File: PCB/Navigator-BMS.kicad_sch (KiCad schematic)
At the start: 49 parts, among them IC1 AP2112K, J1 Conn_01x03, J2 CAN, J3 CAN, J4 Conn_01x05, Q1 IRF7480M, U1 BQ76920PW, U2 MCP2551-I-SN, U3 TMP117xxDRV, U4 STM32G441KBUx, U5 SN74AUP1T34DCK, U6 TPS

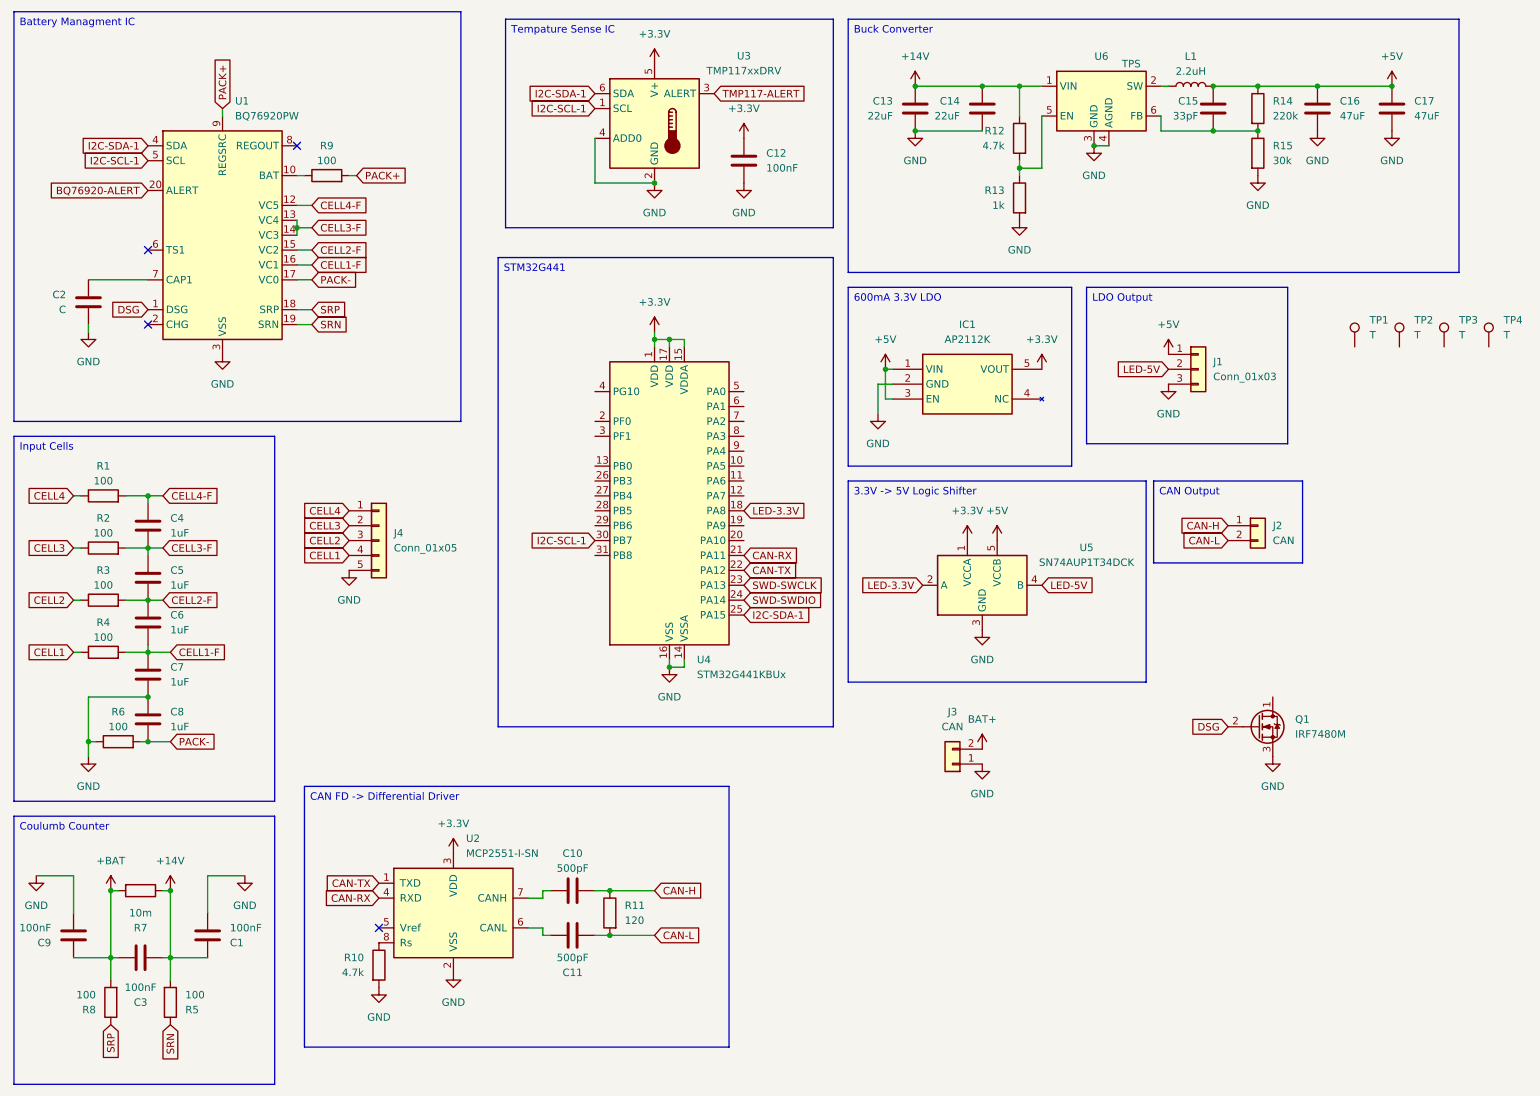
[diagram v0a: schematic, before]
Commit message: Layout Considerations + Schematic almost done
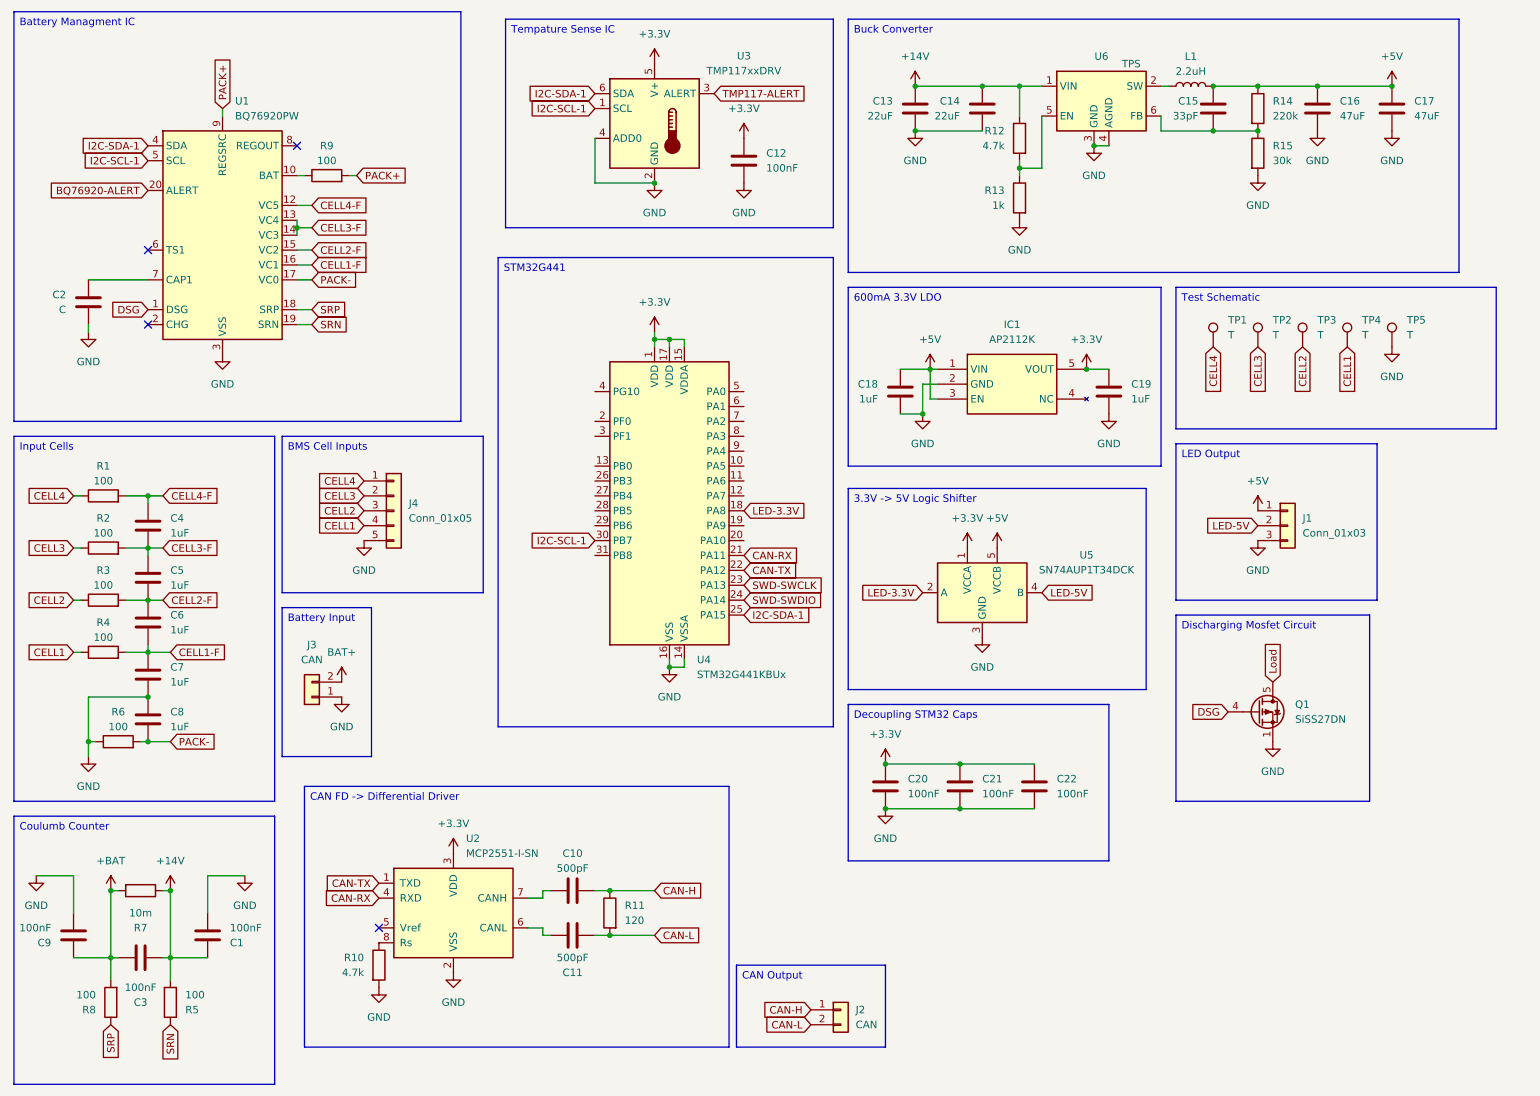
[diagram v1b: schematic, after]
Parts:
- removed Q1: IRF7480M, Package_DirectFET:DirectFET_ME, symbol Transistor_FET:IRF7480M
- added C18, C19: 1uF, Capacitor_SMD:C_0402_1005Metric, symbol Device:C
- added C20, C21, C22: 100nF, Capacitor_SMD:C_0402_1005Metric, symbol Device:C
- added Q1: SiSS27DN, Package_SO:Vishay_PowerPAK_1212-8_Single, symbol Transistor_FET:SiSS27DN
- added TP5: T, TestPoint:TestPoint_Pad_1.0x1.0mm, symbol Connector:TestPoint
- C16, C17: footprint Capacitor_SMD:C_1206_3216Metric -> Capacitor_SMD:C_0805_2012Metric
- J4: footprint (none) -> Connector_JST:JST_EH_B5B-EH-A_1x05_P2.50mm_Vertical
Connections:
- net +3.3V: now also C19.1, C20.1, C21.1, C22.1
- net +5V: now also C18.1
- net CELL1: now also TP4.1
- net CELL2: now also TP3.1
- net CELL3: now also TP2.1
- net CELL4: now also TP1.1
- net DSG: now also Q1.4 (G)
- net GND: now also C18.2, C19.2, C20.2, C21.2, C22.2, Q1.1 (S), Q1.2 (S), Q1.3 (S), TP5.1
- new net Load: Q1.5 (D)
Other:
- moved on the sheet: IC1, J1, J2, J3, J4, TP1, TP2, TP3, TP4, U5
